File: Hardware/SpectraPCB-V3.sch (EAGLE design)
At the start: 35 parts, among them IC1 L293D, IC2 MCP601OT, J1 POWER_JACK, J2 AVR_SPI_PROG_3X2NS, U1 MCP73831

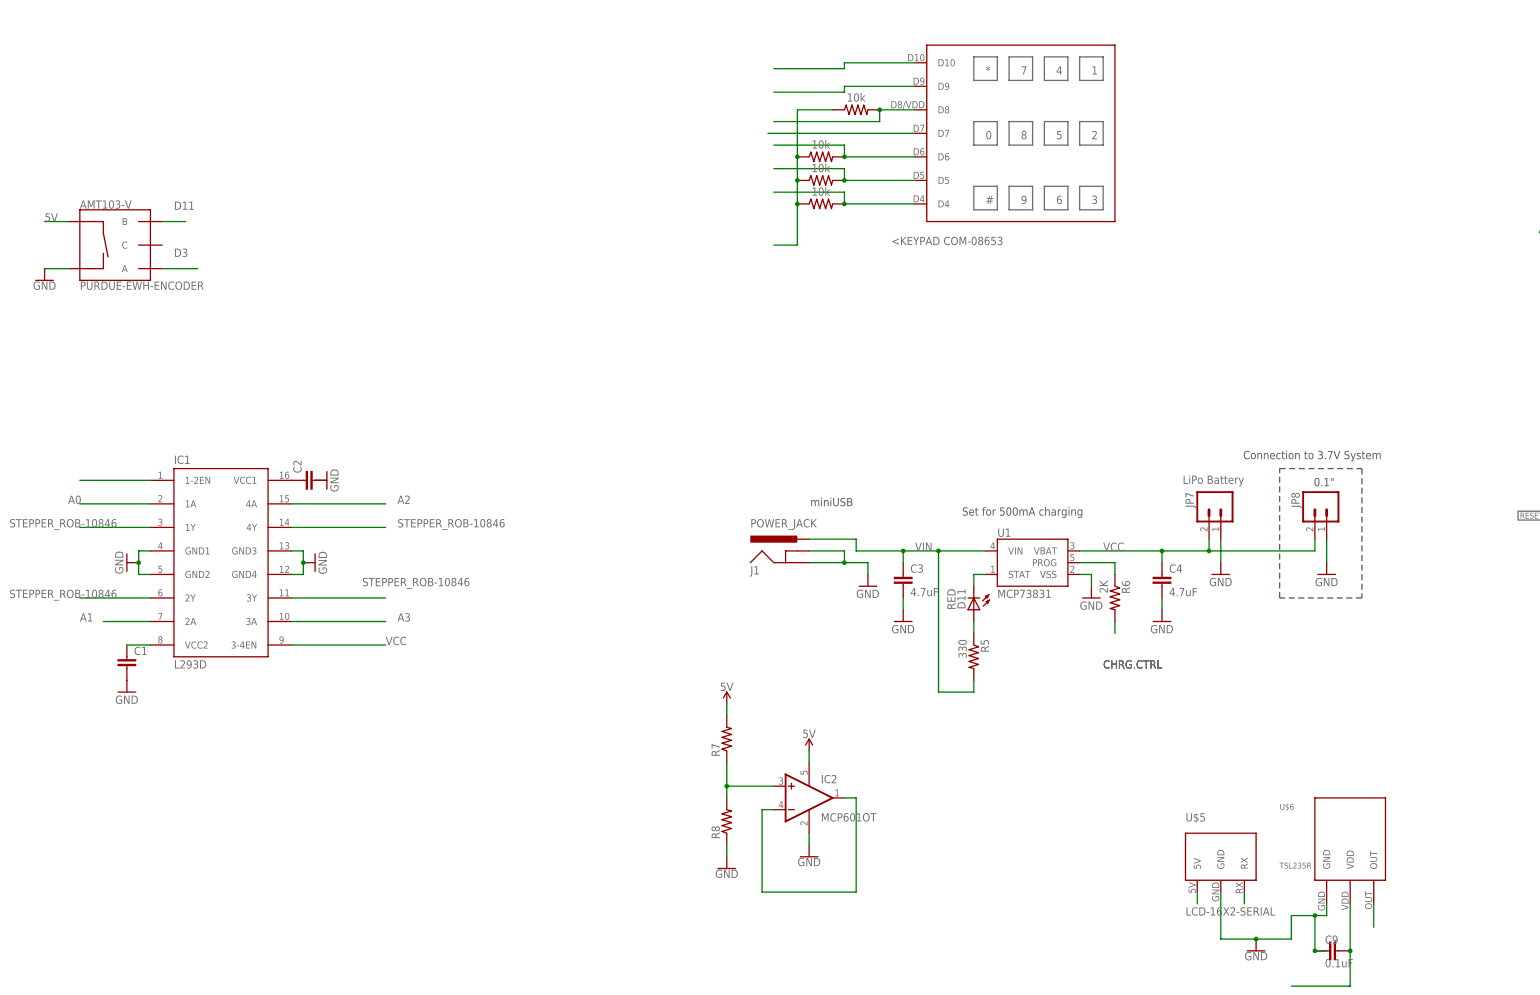
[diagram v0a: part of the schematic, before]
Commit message: Updated SpectaPCB-V3
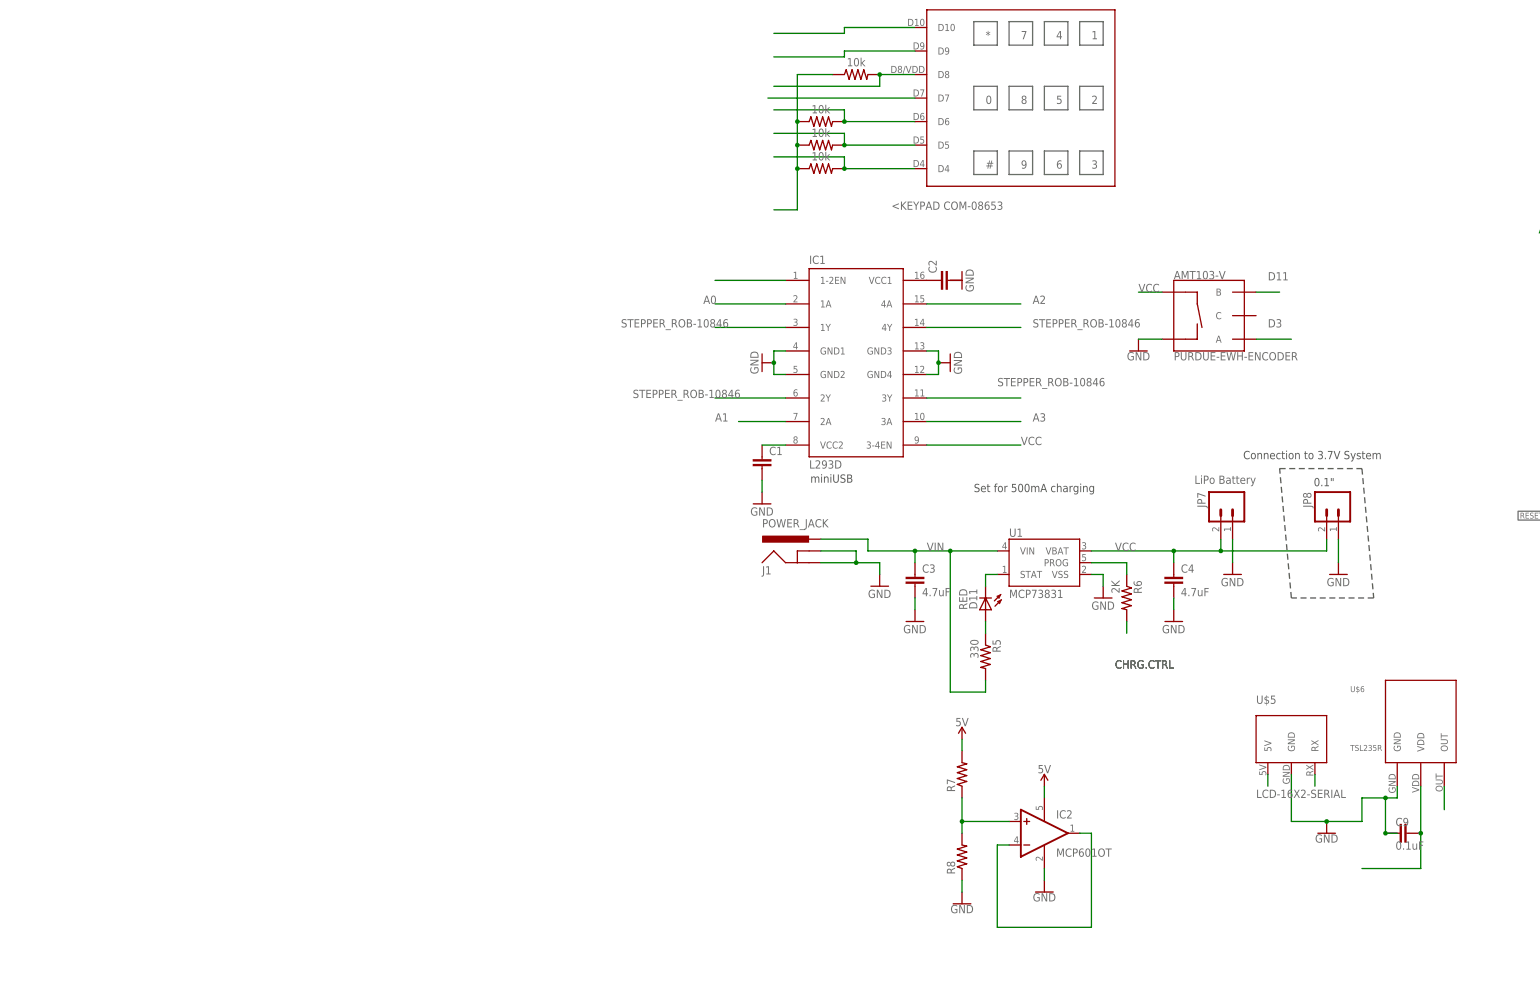
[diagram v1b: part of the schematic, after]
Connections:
- net 5V: no longer AMT103-V.SW+, C9.2, U$6.VDD
- net VCC: now also AMT103-V.SW+, C9.2, U$6.VDD
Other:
- moved on the sheet: AMT103-V, C1, C2, C3, C4, C9, D11, IC1, IC2, J1, JP7, JP8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
